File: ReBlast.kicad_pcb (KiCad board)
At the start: 2 copper layers, 50.7 x 64.9 mm, 23 parts, among them J1 MOS_8580_Socket, U1 74HC20, U2 74HC139, U3 ZN428E-8, U4 TLC272, U5 MOS_8580, U6 ADC0804

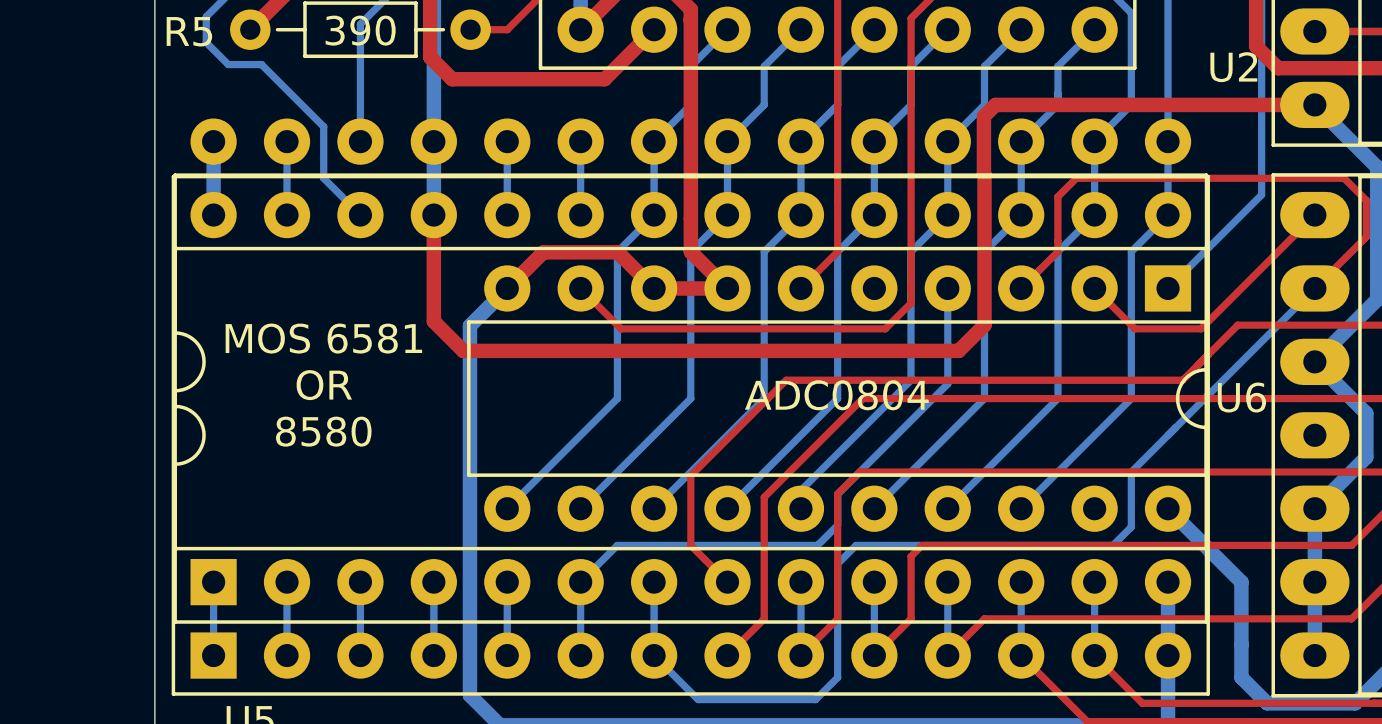
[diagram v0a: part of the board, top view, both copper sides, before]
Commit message: Fix socket
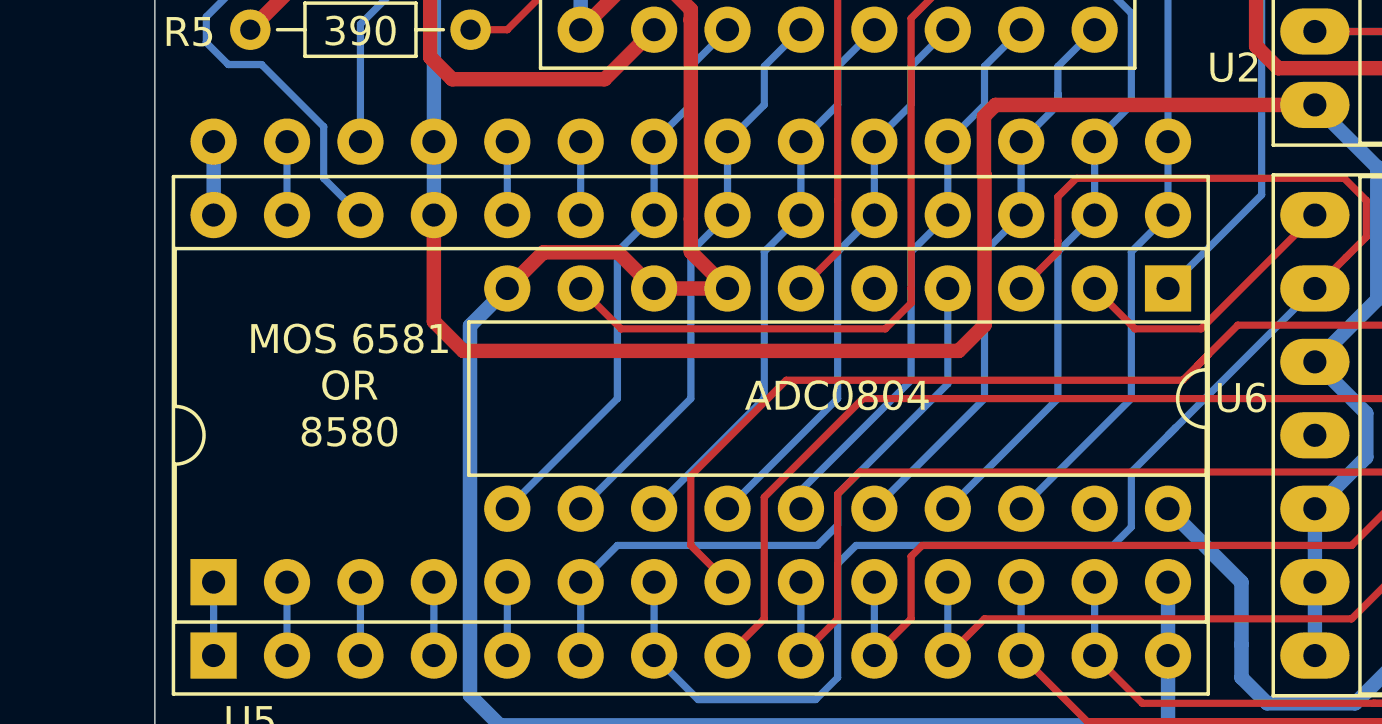
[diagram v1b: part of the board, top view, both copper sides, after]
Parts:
- J1: footprint Package_DIP:DIP-28_W15.24mm -> ReBlast:DIP-28_W15.24mm_Socket
